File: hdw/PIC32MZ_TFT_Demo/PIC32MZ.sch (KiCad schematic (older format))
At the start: 1 part, among them U601 PIC32MZ2048EFG100_IPT

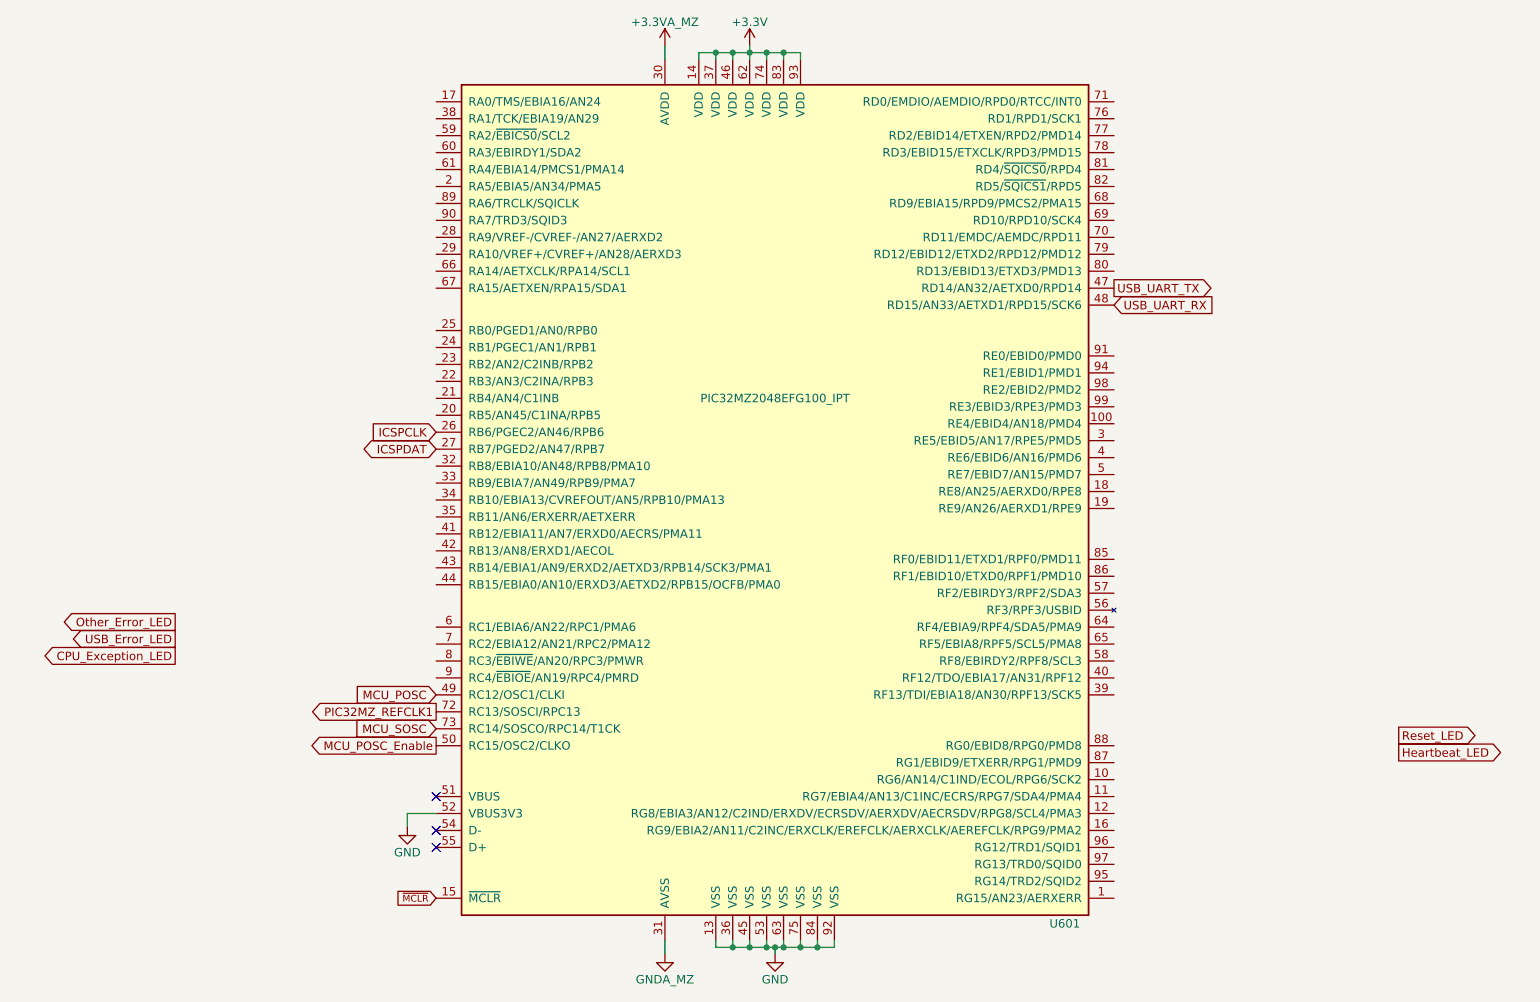
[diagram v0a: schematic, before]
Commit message: Started PCB layout
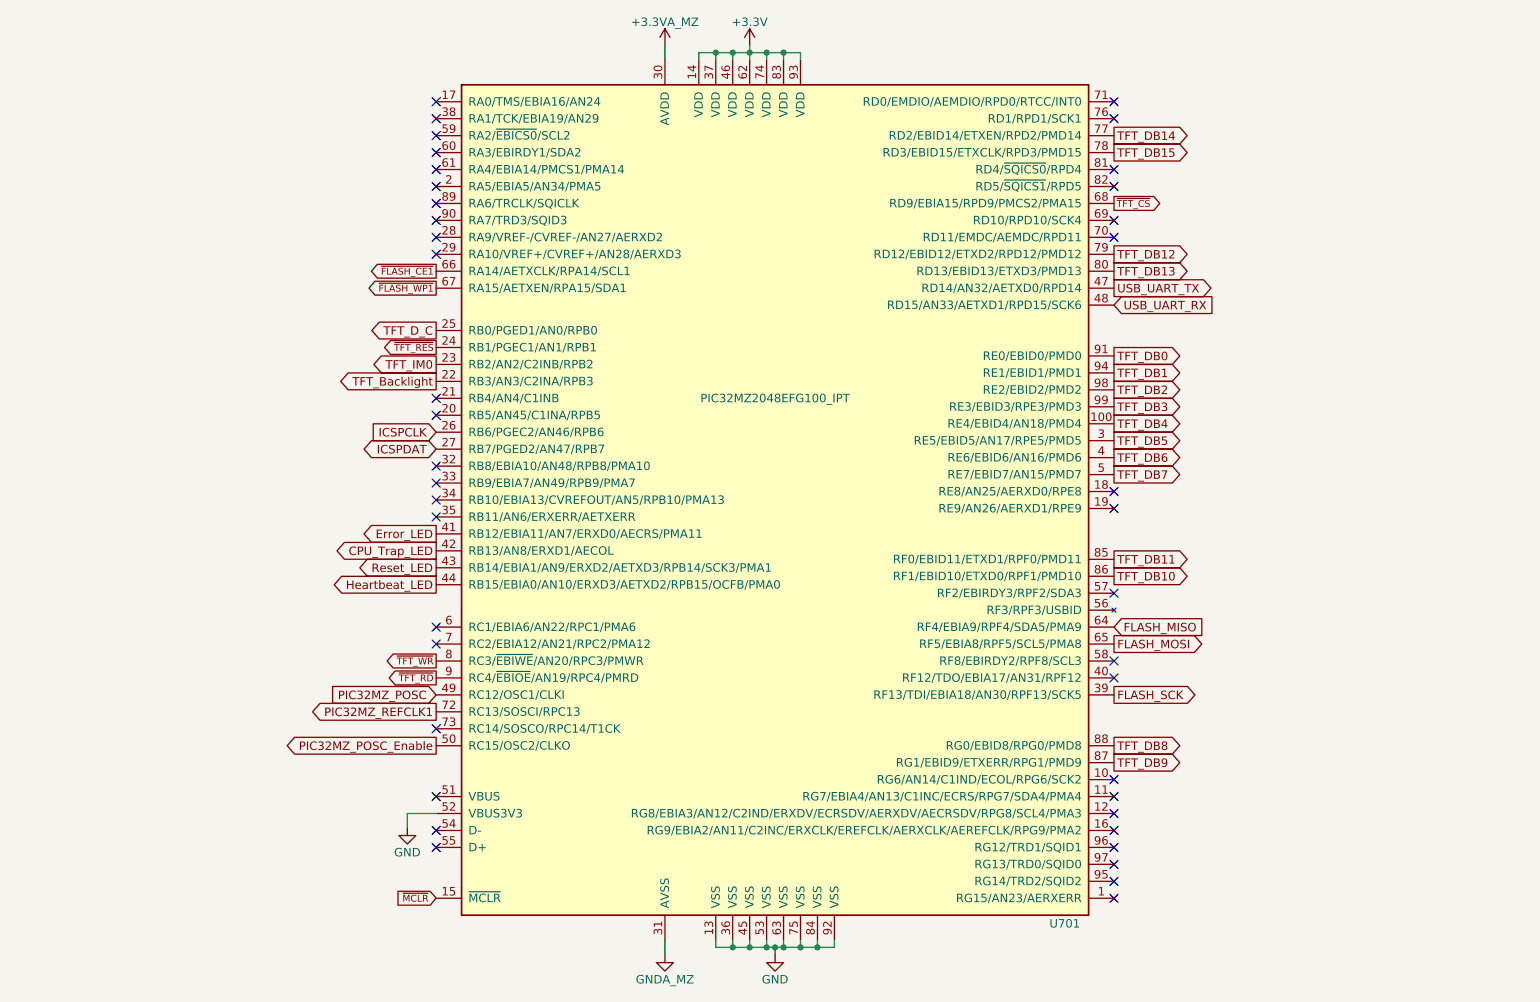
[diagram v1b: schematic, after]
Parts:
- U701: renamed from U601; Digi-Key PN PIC32MZ2048EFG100-I/PT-ND -> PIC32MZ2048EFH100-I/PF-ND
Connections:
- net Heartbeat_LED: now also U701.44 (RB15/EBIA0/AN10/ERXD3/AETXD2/RPB15/OCFB/PMA0)
- net Reset_LED: now also U701.43 (RB14/EBIA1/AN9/ERXD2/AETXD3/RPB14/SCK3/PMA1)
- net TFT_DB4: now reaches U701.100 (RE4/EBID4/AN18/PMD4)
- net TFT_Backlight: now reaches U701.22 (RB3/AN3/C2INA/RPB3)
- net TFT_IM0: now reaches U701.23 (RB2/AN2/C2INB/RPB2)
- net ~TFT_RES: now reaches U701.24 (RB1/PGEC1/AN1/RPB1)
- net TFT_D_C: now reaches U701.25 (RB0/PGED1/AN0/RPB0)
- net TFT_DB5: now reaches U701.3 (RE5/EBID5/AN17/RPE5/PMD5)
- net FLASH_SCK: now reaches U701.39 (RF13/TDI/EBIA18/AN30/RPF13/SCK5)
- net TFT_DB6: now reaches U701.4 (RE6/EBID6/AN16/PMD6)
- net Error_LED: now reaches U701.41 (RB12/EBIA11/AN7/ERXD0/AECRS/PMA11)
- net CPU_Trap_LED: now reaches U701.42 (RB13/AN8/ERXD1/AECOL)
- net TFT_DB7: now reaches U701.5 (RE7/EBID7/AN15/PMD7)
- net FLASH_MISO: now reaches U701.64 (RF4/EBIA9/RPF4/SDA5/PMA9)
- net FLASH_MOSI: now reaches U701.65 (RF5/EBIA8/RPF5/SCL5/PMA8)
- net ~FLASH_CE1: now reaches U701.66 (RA14/AETXCLK/RPA14/SCL1)
- net ~FLASH_WP1: now reaches U701.67 (RA15/AETXEN/RPA15/SDA1)
- net ~TFT_CS: now reaches U701.68 (RD9/EBIA15/RPD9/PMCS2/PMA15)
- net TFT_DB14: now reaches U701.77 (RD2/EBID14/ETXEN/RPD2/PMD14)
- net TFT_DB15: now reaches U701.78 (RD3/EBID15/ETXCLK/RPD3/PMD15)
- net TFT_DB12: now reaches U701.79 (RD12/EBID12/ETXD2/RPD12/PMD12)
- net ~TFT_WR: now reaches U701.8 (RC3/~EBIWE~/AN20/RPC3/PMWR)
- net TFT_DB13: now reaches U701.80 (RD13/EBID13/ETXD3/PMD13)
- net TFT_DB11: now reaches U701.85 (RF0/EBID11/ETXD1/RPF0/PMD11)
- net TFT_DB10: now reaches U701.86 (RF1/EBID10/ETXD0/RPF1/PMD10)
- net TFT_DB9: now reaches U701.87 (RG1/EBID9/ETXERR/RPG1/PMD9)
- net TFT_DB8: now reaches U701.88 (RG0/EBID8/RPG0/PMD8)
- net ~TFT_RD: now reaches U701.9 (RC4/~EBIOE~/AN19/RPC4/PMRD)
- net TFT_DB0: now reaches U701.91 (RE0/EBID0/PMD0)
- net TFT_DB1: now reaches U701.94 (RE1/EBID1/PMD1)
- net TFT_DB2: now reaches U701.98 (RE2/EBID2/PMD2)
- net TFT_DB3: now reaches U701.99 (RE3/EBID3/RPE3/PMD3)
- net MCU_POSC renamed PIC32MZ_POSC
- net MCU_POSC_Enable renamed PIC32MZ_POSC_Enable
- net MCU_SOSC: no longer names the net of U701.73 (RC14/SOSCO/RPC14/T1CK)
- no-connect marks 3 -> 41
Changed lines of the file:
@@
 EESchema Schematic File Version 4
+LIBS:PIC32MZ_TFT_Demo-cache
 EELAYER 30 0
 EELAYER END
 $Descr A 11000 8500
 encoding utf-8
-Sheet 7 11
-Title "VFD Clock"
-Date "2019-04-11"
+Sheet 7 13
+Title ""
+Date "2020-07-04"
 Rev "A"
 Comp "Drew Maatman"
@@
 	5510 920  5410 920
 $Comp
-L power:GND #PWR0605
+L power:GND #PWR0705
 U 1 1 5CB03EF2
 P 5460 6240
-F 0 "#PWR0605" H 5460 5990 50  0001 C CNN
+F 0 "#PWR0705" H 5460 5990 50  0001 C CNN
 F 1 "GND" H 5460 6090 50  0000 C CNN
 F 2 "" H 5460 6240 50  0001 C CNN
@@
 NoConn ~ 3460 5310
 $Comp
-L power:GND #PWR0601
+L power:GND #PWR0701
 U 1 1 5CB14B21
 P 3290 5490
-F 0 "#PWR0601" H 3290 5240 50  0001 C CNN
+F 0 "#PWR0701" H 3290 5240 50  0001 C CNN
 F 1 "GND" H 3290 5340 50  0000 C CNN
 F 2 "" H 3290 5490 50  0001 C CNN
@@
 	3290 5410 3460 5410
 Text GLabel 3460 4710 0    50   Input ~ 0
-MCU_POSC
-Text GLabel 3460 4910 0    50   Input ~ 0
-MCU_SOSC
+PIC32MZ_POSC
 Text GLabel 3460 3260 0    50   BiDi ~ 0
 ICSPDAT
@@
 ICSPCLK
 Text GLabel 3460 5010 0    50   Output ~ 0
-MCU_POSC_Enable
+PIC32MZ_POSC_Enable
 Text GLabel 7460 2410 2    50   Input ~ 0
 USB_UART_RX
@@
 USB_UART_TX
 $Comp
-L Custom_Library:PIC32MZ2048EFG100_IPT U601
+L Custom_Library:PIC32MZ2048EFG100_IPT U701
 U 1 1 5E6CE439
 P 5460 3560
-F 0 "U601" H 7260 1060 50  0000 R CNN
+F 0 "U701" H 7260 1060 50  0000 R CNN
 F 1 "PIC32MZ2048EFG100_IPT" H 5460 4160 50  0000 C CNN
 F 2 "Housings_QFP:TQFP-100_14x14mm_Pitch0.5mm" H 5460 3560 50  0001 C CNN
 F 3 "http://ww1.microchip.com/downloads/en/DeviceDoc/60001320E.pdf" H 5460 3560 50  0001 C CNN
 F 4 "ALL" H 5460 3560 50  0001 C CNN "Config"
-F 5 "PIC32MZ2048EFG100-I/PT-ND" H 5460 3560 50  0001 C CNN "Digi-Key PN"
+F 5 "PIC32MZ2048EFH100-I/PF-ND" H 5460 3560 50  0001 C CNN "Digi-Key PN"
 	1    5460 3560
 	1    0    0    -1
 $EndComp
 $Comp
-L power:+3.3V #PWR0604
+L power:+3.3V #PWR0704
 U 1 1 5E6E7B25
 P 5310 880
-F 0 "#PWR0604" H 5310 730 50  0001 C CNN
+F 0 "#PWR0704" H 5310 730 50  0001 C CNN
 F 1 "+3.3V" H 5310 1020 50  0000 C CNN
 F 2 "" H 5310 880 50  0001 C CNN
@@
 	1    0    0    -1
 $EndComp
-Text GLabel 9140 5050 2    50   Output ~ 0
+Text GLabel 3460 4060 0    50   Output ~ 0
 Heartbeat_LED
-Text GLabel 9140 4950 2    50   Output ~ 0
+Text GLabel 3460 3960 0    50   Output ~ 0
 Reset_LED
-Text GLabel 1920 4380 0    50   Output ~ 0
-USB_Error_LED
-Text GLabel 1920 4280 0    50   Output ~ 0
-Other_Error_LED
-Text GLabel 1920 4480 0    50   Output ~ 0
-CPU_Exception_LED
-$Comp
-L Custom_Library:GNDA_MZ #PWR?
+Text GLabel 3460 3760 0    50   Output ~ 0
+Error_LED
+Text GLabel 3460 3860 0    50   Output ~ 0
+CPU_Trap_LED
+$Comp
+L Custom_Library:GNDA_MZ #PWR0703
 U 1 1 5EE47433
 P 4810 6240
-F 0 "#PWR?" H 4810 5990 50  0001 C CNN
+F 0 "#PWR0703" H 4810 5990 50  0001 C CNN
 F 1 "GNDA_MZ" H 4810 6090 50  0000 C CNN
 F 2 "" H 4810 6240 50  0001 C CNN
@@
 $EndComp
 $Comp
-L Custom_Library:+3.3VA_MZ #PWR?
+L Custom_Library:+3.3VA_MZ #PWR0702
 U 1 1 5EE478C2
 P 4810 880
-F 0 "#PWR?" H 4810 730 50  0001 C CNN
+F 0 "#PWR0702" H 4810 730 50  0001 C CNN
 F 1 "+3.3VA_MZ" H 4810 1020 50  0000 C CNN
 F 2 "" H 4810 880 50  0001 C CNN
@@
 Text GLabel 3460 4810 0    50   Output ~ 0
 PIC32MZ_REFCLK1
+Text GLabel 7460 1810 2    40   Output ~ 0
+~TFT_CS
+Text GLabel 3460 2560 0    50   Output ~ 0
+TFT_D_C
+Text GLabel 3460 4510 0    40   Output ~ 0
+~TFT_WR
+Text GLabel 3460 4610 0    40   Output ~ 0
+~TFT_RD
+Text GLabel 7460 2710 2    50   Output ~ 0
+TFT_DB0
+Text GLabel 7460 2810 2    50   Output ~ 0
+TFT_DB1
+Text GLabel 7460 2910 2    50   Output ~ 0
+TFT_DB2
+Text GLabel 7460 3010 2    50   Output ~ 0
+TFT_DB3
+Text GLabel 7460 3110 2    50   Output ~ 0
+TFT_DB4
+Text GLabel 7460 3210 2    50   Output ~ 0
+TFT_DB5
+Text GLabel 7460 3310 2    50   Output ~ 0
+TFT_DB6
+Text GLabel 7460 3410 2    50   Output ~ 0
+TFT_DB7
+Text GLabel 7460 5010 2    50   Output ~ 0
+TFT_DB8
+Text GLabel 7460 5110 2    50   Output ~ 0
+TFT_DB9
+Text GLabel 7460 4010 2    50   Output ~ 0
+TFT_DB10
+Text GLabel 7460 3910 2    50   Output ~ 0
+TFT_DB11
+Text GLabel 7460 2110 2    50   Output ~ 0
+TFT_DB12
+Text GLabel 7460 2210 2    50   Output ~ 0
+TFT_DB13
+Text GLabel 7460 1410 2    50   Output ~ 0
+TFT_DB14
+Text GLabel 7460 1510 2    50   Output ~ 0
+TFT_DB15
+Text GLabel 3460 2660 0    40   Output ~ 0
+~TFT_RES
+Text GLabel 3460 2760 0    50   Output ~ 0
+TFT_IM0
+Text GLabel 7460 4710 2    50   Output ~ 0
+FLASH_SCK
+Text GLabel 3460 2210 0    40   Output ~ 0
+~FLASH_CE1
+Text GLabel 7460 4410 2    50   Output ~ 0
+FLASH_MOSI
+Text GLabel 3460 2310 0    40   Output ~ 0
+~FLASH_WP1
+Text GLabel 7460 4310 2    50   Input ~ 0
+FLASH_MISO
+Text GLabel 3460 2860 0    50   Output ~ 0
+TFT_Backlight
+NoConn ~ 3460 1210
+NoConn ~ 3460 1310
+NoConn ~ 3460 1410
+NoConn ~ 3460 1510
+NoConn ~ 3460 1610
+NoConn ~ 3460 1710
+NoConn ~ 3460 1810
+NoConn ~ 3460 1910
+NoConn ~ 3460 2010
+NoConn ~ 3460 2110
+NoConn ~ 3460 2960
+NoConn ~ 3460 3060
+NoConn ~ 3460 3360
+NoConn ~ 3460 3460
+NoConn ~ 3460 3560
+NoConn ~ 3460 3660
+NoConn ~ 3460 4310
+NoConn ~ 3460 4410
+NoConn ~ 7460 1210
+NoConn ~ 7460 1310
+NoConn ~ 7460 1610
+NoConn ~ 7460 1710
+NoConn ~ 7460 1910
+NoConn ~ 7460 2010
+NoConn ~ 7460 3510
+NoConn ~ 7460 3610
+NoConn ~ 3460 4910
+NoConn ~ 7460 4110
+NoConn ~ 7460 4510
+NoConn ~ 7460 4610
+NoConn ~ 7460 5210
+NoConn ~ 7460 5310
+NoConn ~ 7460 5410
+NoConn ~ 7460 5510
+NoConn ~ 7460 5610
+NoConn ~ 7460 5710
+NoConn ~ 7460 5810
+NoConn ~ 7460 5910
 $EndSCHEMATC
